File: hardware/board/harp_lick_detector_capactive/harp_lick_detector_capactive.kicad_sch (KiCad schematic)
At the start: 46 parts

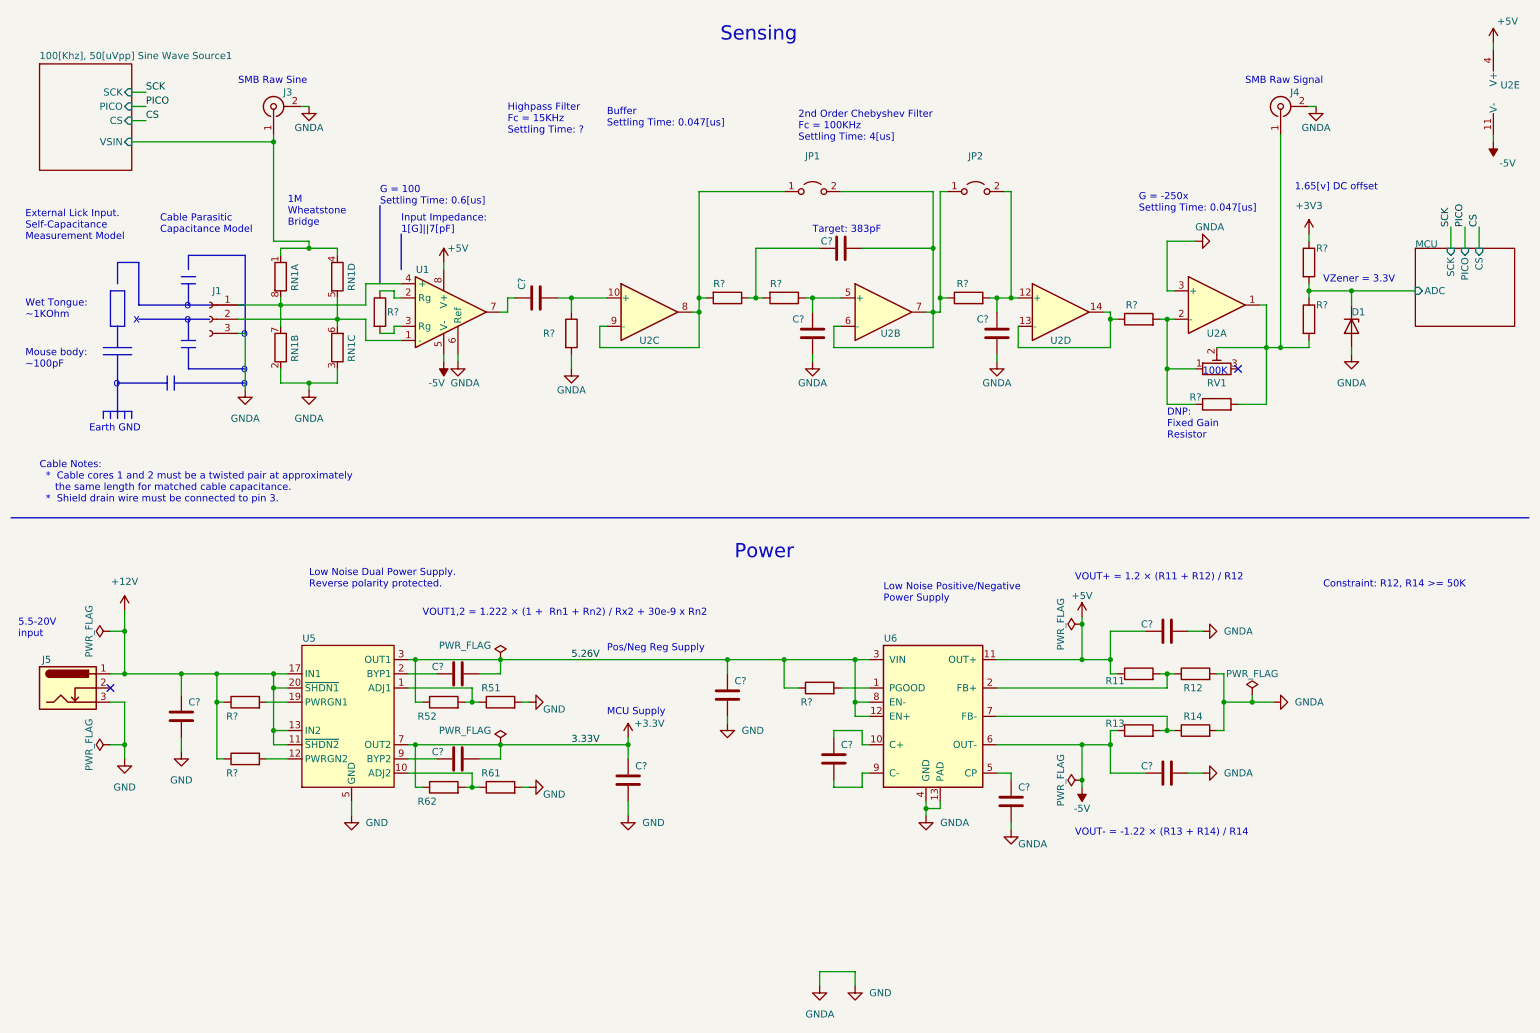
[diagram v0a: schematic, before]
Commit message: complete bom draft
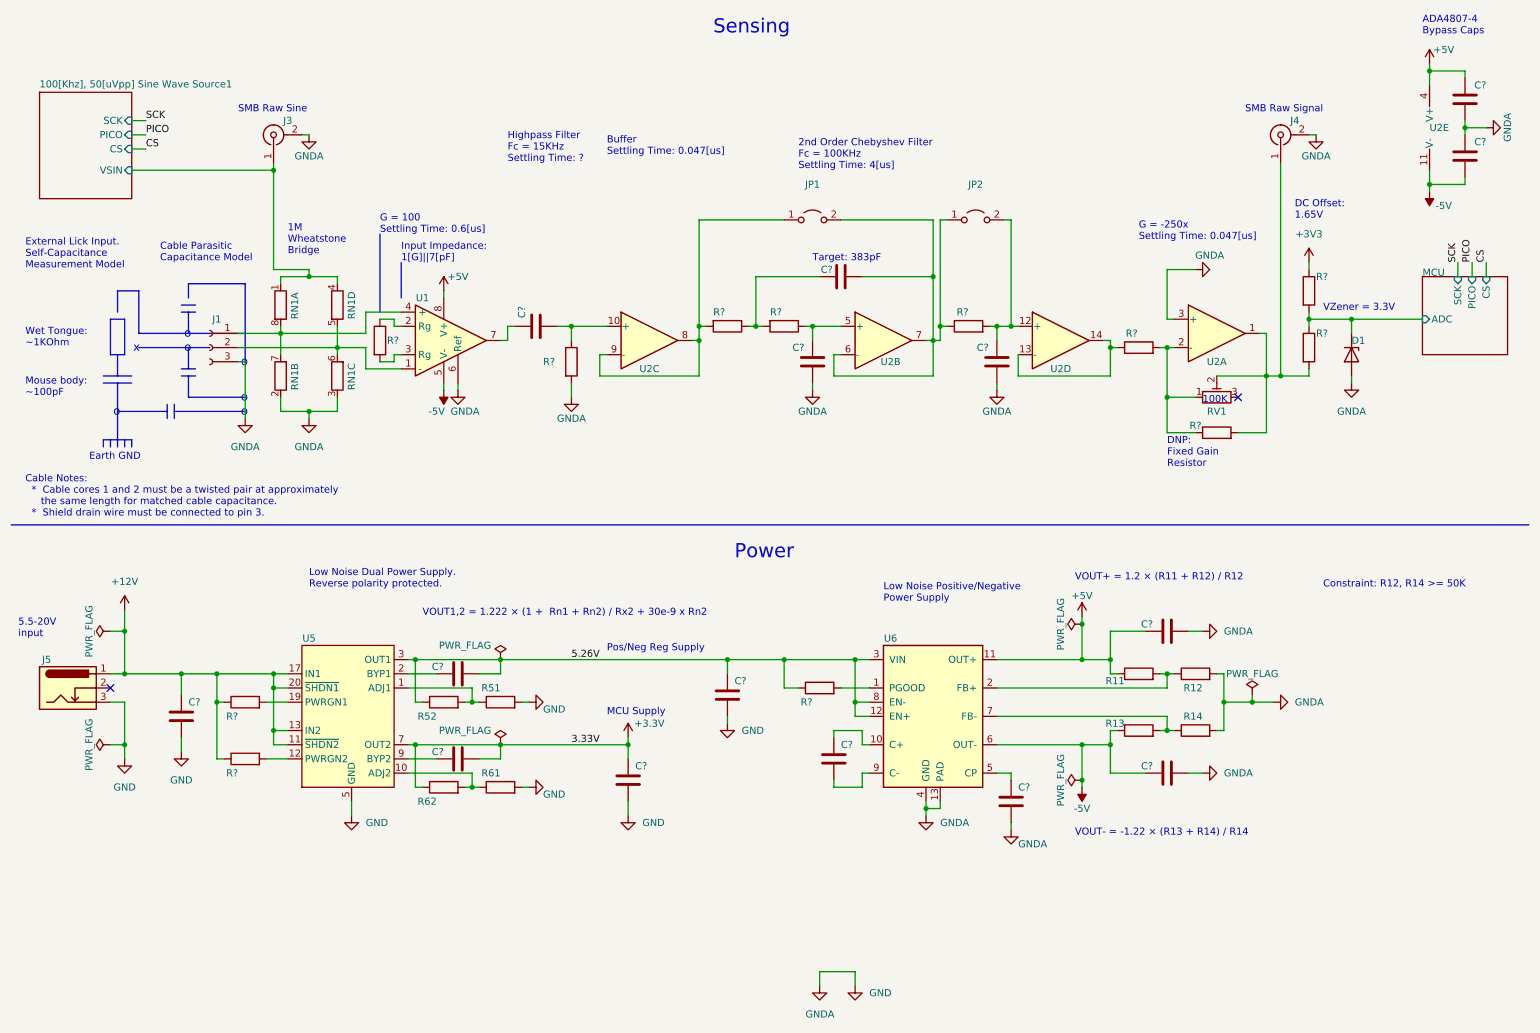
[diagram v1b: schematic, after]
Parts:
- added C? (x2): (no value), symbol Device:C
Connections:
- net +5V: now also C?.2
- net -5V: now also C?.1
- net GND: now also C?.1, C?.2
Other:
- note added: "ADA4807-4 Bypass Caps"
- note added: "DC Offset: 1.65V"
- note removed: "1.65[v] DC offset"
- moved on the sheet: C?, D1, J1, J3, J4, JP1, JP2, R?, RN1A, RN1B, RN1C, RN1D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
